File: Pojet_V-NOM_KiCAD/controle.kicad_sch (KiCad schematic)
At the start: 0 parts

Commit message: Mise à jour du schéma éléctrique
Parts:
- added IC1: STM32G431CBU6, QFN50P700X700X65-49N-D, symbol STM32G431CBU6:STM32G431CBU6
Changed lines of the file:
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@@
 	(generator_version "8.0")
 	(paper "A4")
+	(symbol
+		(lib_id "STM32G431CBU6:STM32G431CBU6")
+		(at 123.19 87.63 0)
+		(unit 1)
+		(exclude_from_sim no)
+		(in_bom yes)
+		(on_board yes)
+		(dnp no)
+		(fields_autoplaced yes)
+		(property "Reference" "IC1"
+			(at 172.72 81.3114 0)
+			(effects
+				(font
+					(size 1.27 1.27)
+				)
+			)
+		)
+		(property "Value" "STM32G431CBU6"
+			(at 172.72 83.8514 0)
+			(effects
+				(font
+					(size 1.27 1.27)
+				)
+			)
+		)
+		(property "Footprint" "QFN50P700X700X65-49N-D"
+			(at 165.1 167.31 0)
+			(effects
+				(font
+					(size 1.27 1.27)
+				)
+				(justify left top)
+				(hide yes)
+			)
+		)
+		(property "Datasheet" "https://www.st.com/resource/en/datasheet/stm32g431cb.pdf"
+			(at 165.1 267.31 0)
+			(effects
+				(font
+					(size 1.27 1.27)
+				)
+				(justify left top)
+				(hide yes)
+			)
+		)
+		(property "Description" "STMICROELECTRONICS - STM32G431CBU6 - MCU, 32BIT, 170MHZ, UFQFPN-48"
+			(at 123.19 87.63 0)
+			(effects
+				(font
+					(size 1.27 1.27)
+				)
+				(hide yes)
+			)
+		)
+		(property "Height" "0.65"
+			(at 165.1 467.31 0)
+			(effects
+				(font
+					(size 1.27 1.27)
+				)
+				(justify left top)
+				(hide yes)
+			)
+		)
+		(property "Manufacturer_Name" "STMicroelectronics"
+			(at 165.1 567.31 0)
+			(effects
+				(font
+					(size 1.27 1.27)
+				)
+				(justify left top)
+				(hide yes)
+			)
+		)
+		(property "Manufacturer_Part_Number" "STM32G431CBU6"
+			(at 165.1 667.31 0)
+			(effects
+				(font
+					(size 1.27 1.27)
+				)
+				(justify left top)
+				(hide yes)
+			)
+		)
+		(property "Mouser Part Number" "511-STM32G431CBU6"
+			(at 165.1 767.31 0)
+			(effects
+				(font
+					(size 1.27 1.27)
+				)
+				(justify left top)
+				(hide yes)
+			)
+		)
+		(property "Mouser Price/Stock" "https://www.mouser.co.uk/ProductDetail/STMicroelectronics/STM32G431CBU6?qs=T3oQrply3y%252B0hTuSHQ7oqA%3D%3D"
+			(at 165.1 867.31 0)
+			(effects
+				(font
+					(size 1.27 1.27)
+				)
+				(justify left top)
+				(hide yes)
+			)
+		)
+		(property "Arrow Part Number" "STM32G431CBU6"
+			(at 165.1 967.31 0)
+			(effects
+				(font
+					(size 1.27 1.27)
+				)
+				(justify left top)
+				(hide yes)
+			)
+		)
+		(property "Arrow Price/Stock" "https://www.arrow.com/en/products/stm32g431cbu6/stmicroelectronics?region=nac"
+			(at 165.1 1067.31 0)
+			(effects
+				(font
+					(size 1.27 1.27)
+				)
+				(justify left top)
+				(hide yes)
+			)
+		)
+		(pin "34"
+		)
+		(pin "18"
+		)
+		(pin "45"
+		)
+		(pin "44"
+		)
+		(pin "41"
+		)
+		(pin "8"
+		)
+		(pin "47"
+		)
+		(pin "49"
+		)
+		(pin "20"
+		)
+		(pin "17"
+		)
+		(pin "48"
+		)
+		(pin "46"
+		)
+		(pin "9"
+		)
+		(pin "25"
+		)
+		(pin "30"
+		)
+		(pin "31"
+		)
+		(pin "32"
+		)
+		(pin "36"
+		)
+		(pin "35"
+		)
+		(pin "37"
+		)
+		(pin "39"
+		)
+		(pin "27"
+		)
+		(pin "15"
+		)
+		(pin "4"
+		)
+		(pin "13"
+		)
+		(pin "14"
+		)
+		(pin "38"
+		)
+		(pin "12"
+		)
+		(pin "11"
+		)
+		(pin "10"
+		)
+		(pin "16"
+		)
+		(pin "24"
+		)
+		(pin "33"
+		)
+		(pin "1"
+		)
+		(pin "40"
+		)
+		(pin "5"
+		)
+		(pin "22"
+		)
+		(pin "19"
+		)
+		(pin "3"
+		)
+		(pin "2"
+		)
+		(pin "26"
+		)
+		(pin "23"
+		)
+		(pin "6"
+		)
+		(pin "7"
+		)
+		(pin "29"
+		)
+		(pin "28"
+		)
+		(pin "43"
+		)
+		(pin "21"
+		)
+		(pin "42"
+		)
+		(instances
+			(project ""
+				(path "/37e0fdad-f3fd-48e0-8377-111662233a91/d618a370-a672-4f19-b1d1-7104c075c5ae"
+					(reference "IC1")
+					(unit 1)
+				)
+			)
+		)
+	)
 )

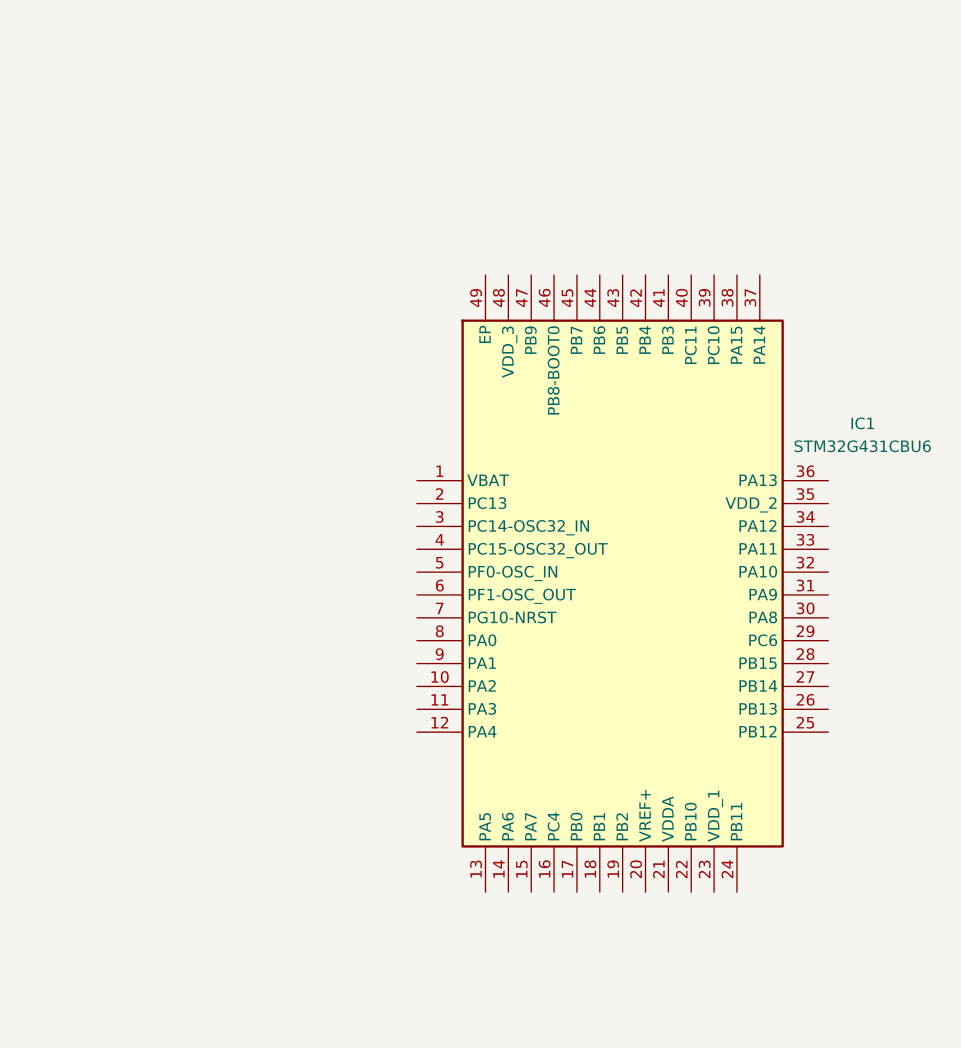
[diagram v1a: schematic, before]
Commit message: Pins configurés projet STM32CubeIDE
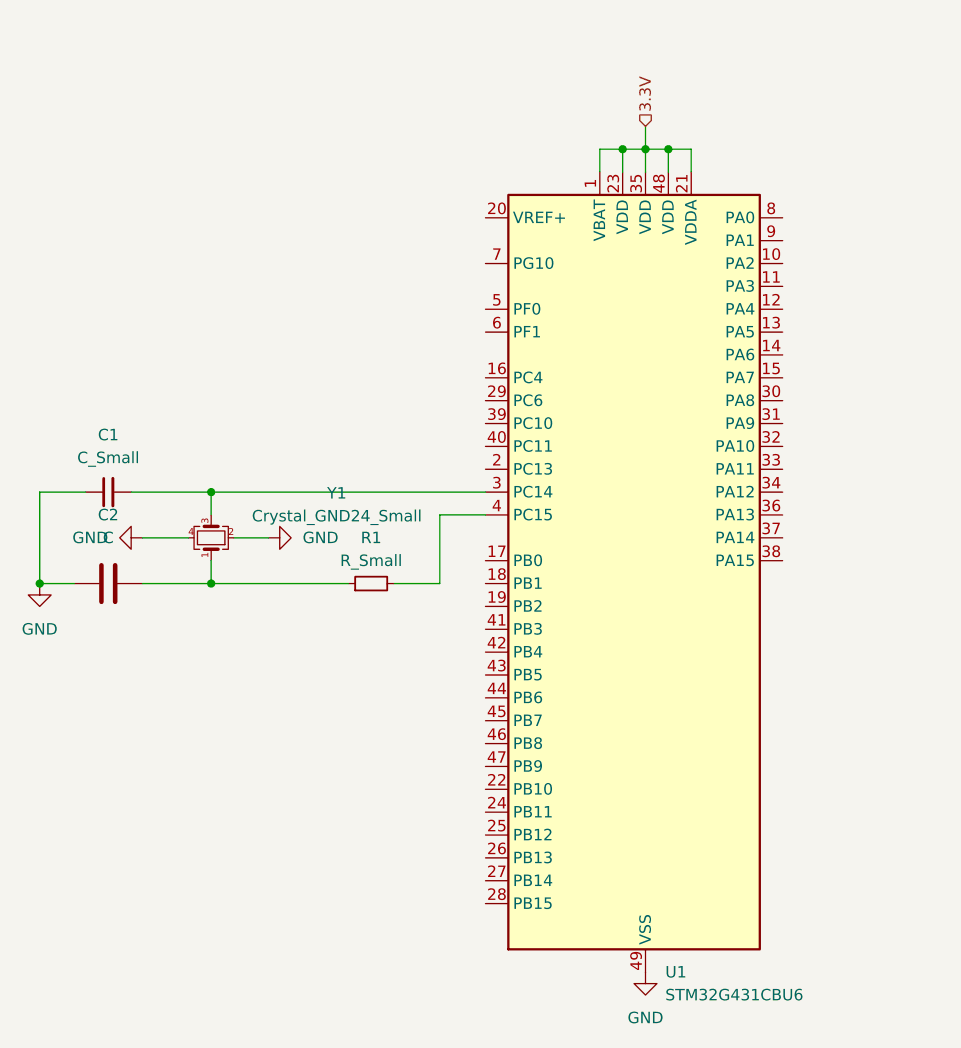
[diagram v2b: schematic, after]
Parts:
- removed IC1: STM32G431CBU6, QFN50P700X700X65-49N-D, symbol STM32G431CBU6:STM32G431CBU6
- added C1: C_Small, symbol Device:C_Small
- added C2: C, symbol Device:C
- added R1: R_Small, symbol Device:R_Small
- added U1: STM32G431CBU6, Package_DFN_QFN:QFN-48-1EP_7x7mm_P0.5mm_EP5.6x5.6mm, symbol MCU_ST_STM32G4:STM32G431CBUx
- added Y1: Crystal_GND24_Small, symbol Device:Crystal_GND24_Small
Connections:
- new net: C1.2, U1.3 (PC14), Y1.3
- new net: R1.2, U1.4 (PC15)
- new net: C2.2, R1.1, Y1.1
- new net 3.3V: U1.1 (VBAT), U1.21 (VDDA), U1.23 (VDD), U1.35 (VDD), U1.48 (VDD)
- new net GND: C1.1, C2.1, U1.49 (VSS), Y1.2, Y1.4

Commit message: Mise à jour des pins
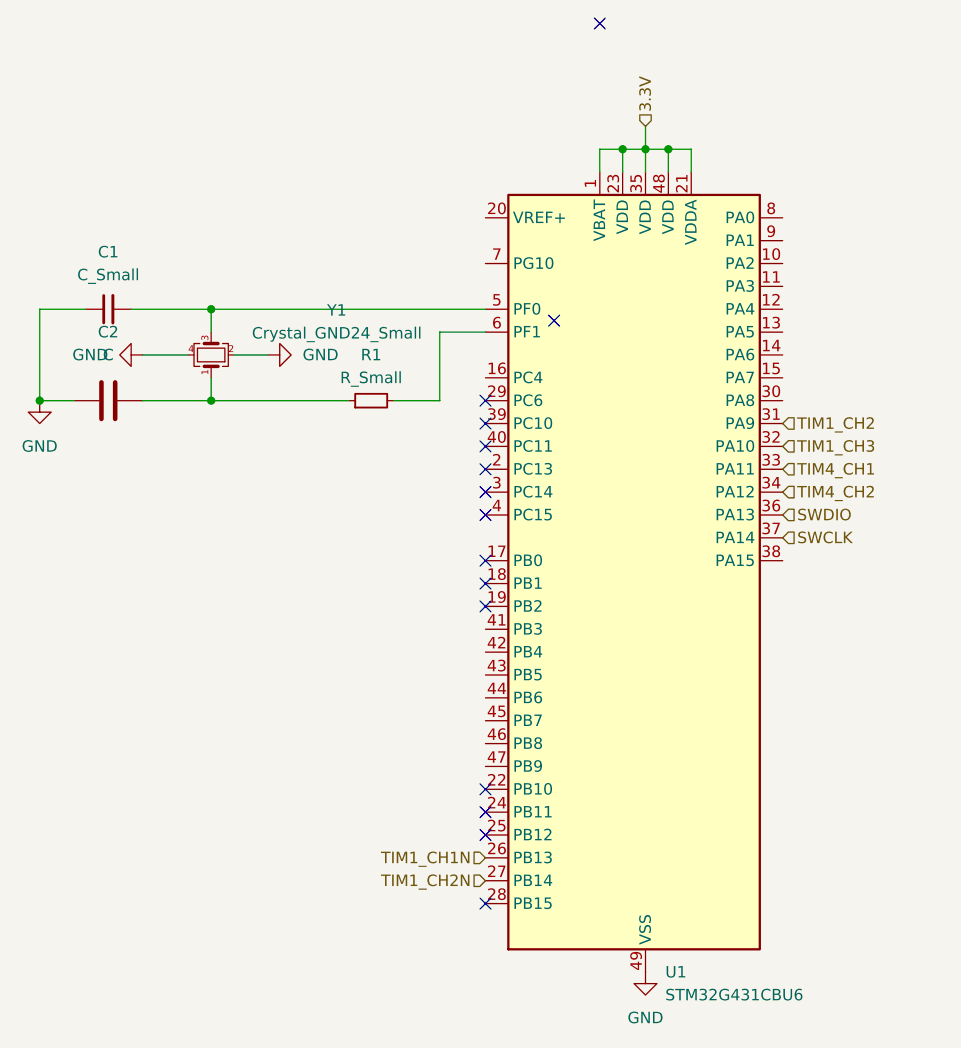
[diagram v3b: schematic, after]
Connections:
- net TIM1_CH1N: now reaches U1.26 (PB13)
- net TIM1_CH2N: now reaches U1.27 (PB14)
- net at C1.2, Y1.3: now also U1.5 (PF0); no longer U1.3 (PC14)
- net TIM1_CH2: now reaches U1.31 (PA9)
- net TIM1_CH3: now reaches U1.32 (PA10)
- net TIM4_CH1: now reaches U1.33 (PA11)
- net TIM4_CH2: now reaches U1.34 (PA12)
- net SWDIO: now reaches U1.36 (PA13)
- net SWCLK: now reaches U1.37 (PA14)
- net at U1.4 (PC15): no longer R1.2
- net at U1.6 (PF1): now also R1.2
- no-connect marks 0 -> 15
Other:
- moved on the sheet: C1, C2, R1, Y1
